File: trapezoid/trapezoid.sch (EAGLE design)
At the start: 30 parts, among them IC2 LGD20H, U1 MMA8452Q, U2 microSD, U4 MCP73831, Y1 CRYSTAL.ABS25

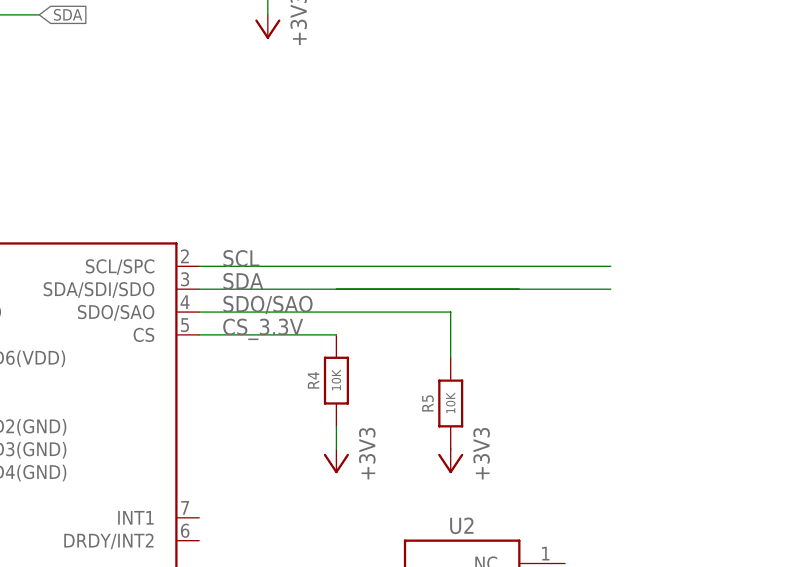
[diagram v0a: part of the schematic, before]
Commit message: placed rtc and usd
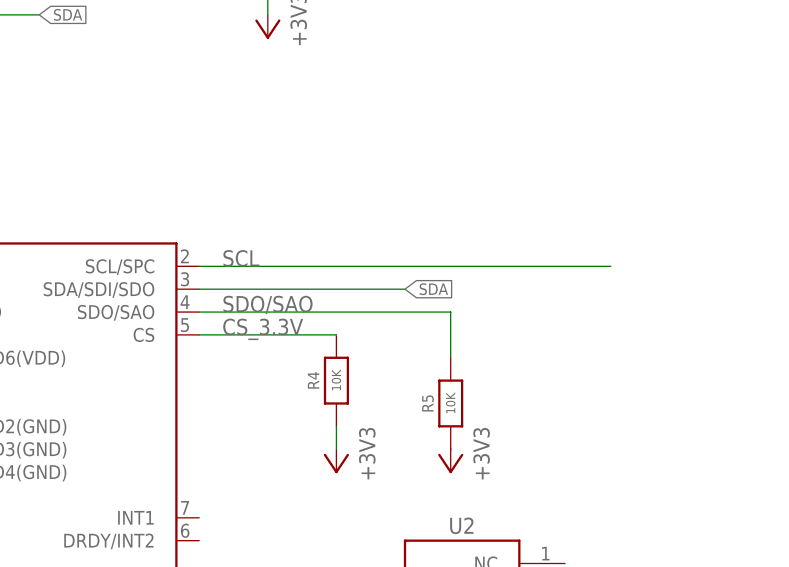
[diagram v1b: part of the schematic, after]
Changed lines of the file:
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@@
-</segment>
-<segment>
-<wire x1="139.7" y1="91.44" x2="185.42" y2="91.44" width="0.1524" layer="91"/>
-<label x="142.24" y="91.44" size="1.778" layer="95"/>
-<pinref part="IC2" gate="G$1" pin="SDA/SDI/SDO"/>
 </segment>
 <segment>
@@
 <wire x1="111.76" y1="121.92" x2="121.92" y2="121.92" width="0.1524" layer="91"/>
 <label x="121.92" y="121.92" size="1.27" layer="95" xref="yes"/>
+</segment>
+<segment>
+<pinref part="IC2" gate="G$1" pin="SDA/SDI/SDO"/>
+<wire x1="139.7" y1="91.44" x2="162.56" y2="91.44" width="0.1524" layer="91"/>
+<label x="162.56" y="91.44" size="1.27" layer="95" xref="yes"/>
 </segment>
 </net>
@@
 </segment>
 </net>
-<net name="N$8" class="0">
-<segment>
-<wire x1="154.94" y1="91.44" x2="175.26" y2="91.44" width="0.1524" layer="91"/>
-</segment>
-</net>
